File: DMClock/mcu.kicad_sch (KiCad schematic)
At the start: 23 parts, among them J7 Conn_01x01_Pin, J8 Conn_01x01_Pin, Q1 2SC1815, Q2 2SC1815, SW1 SW_Push, SW10 SW_Push, SW3 SW_SP3T (mode select), SW7 SW_Push, SW8 SW_Push, SW9 SW_Push, U1 PIC16F18346-P, U2 DS3231SN_

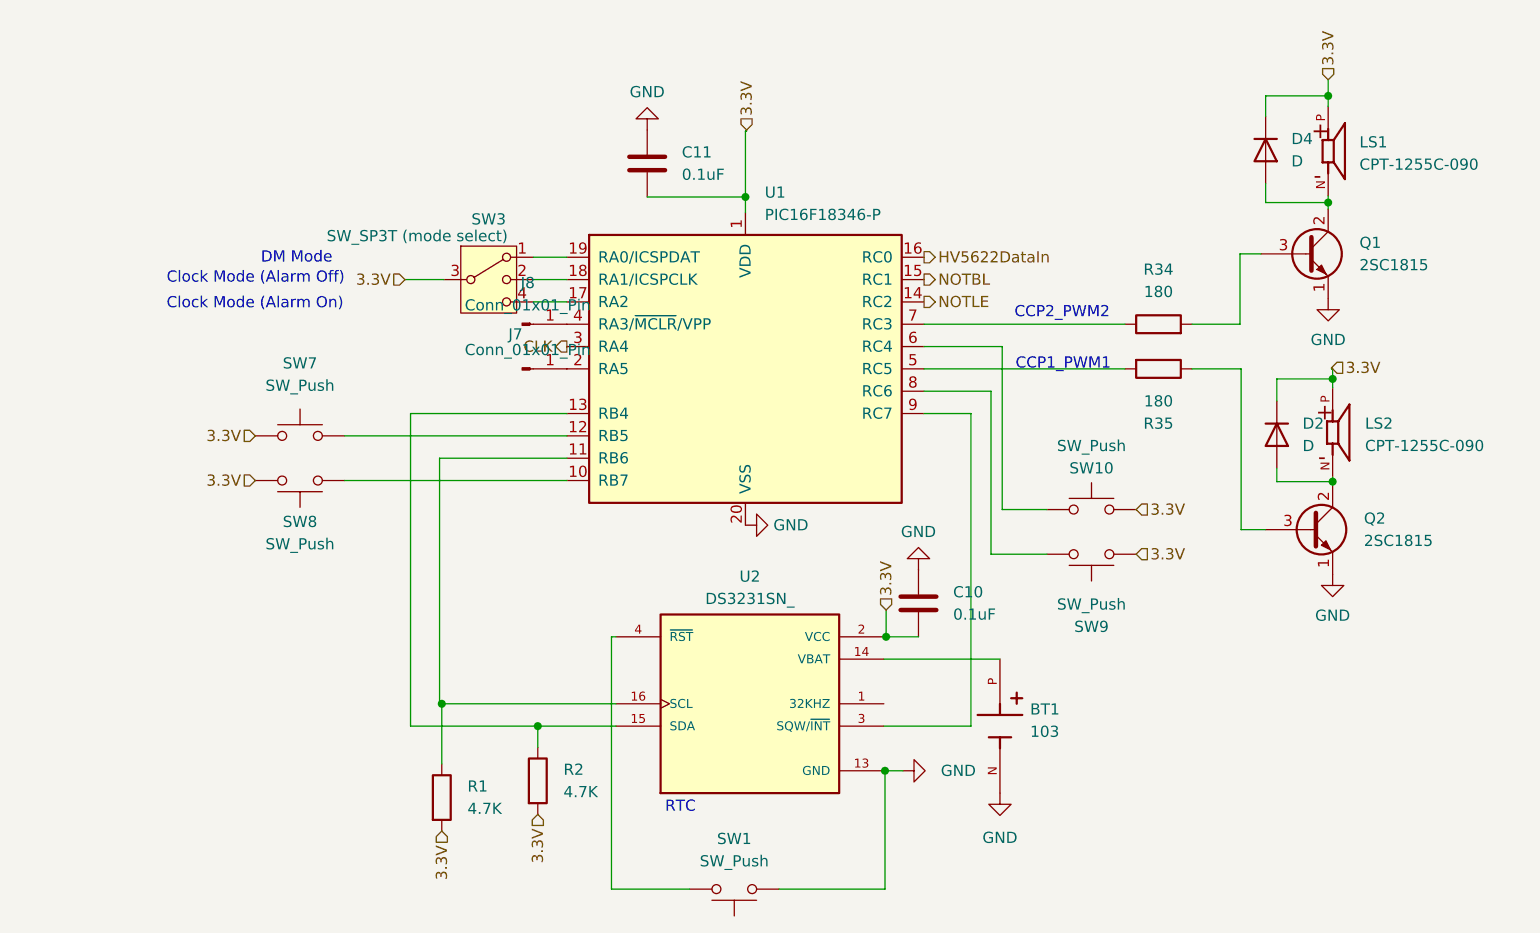
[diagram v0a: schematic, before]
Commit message: finished v.1
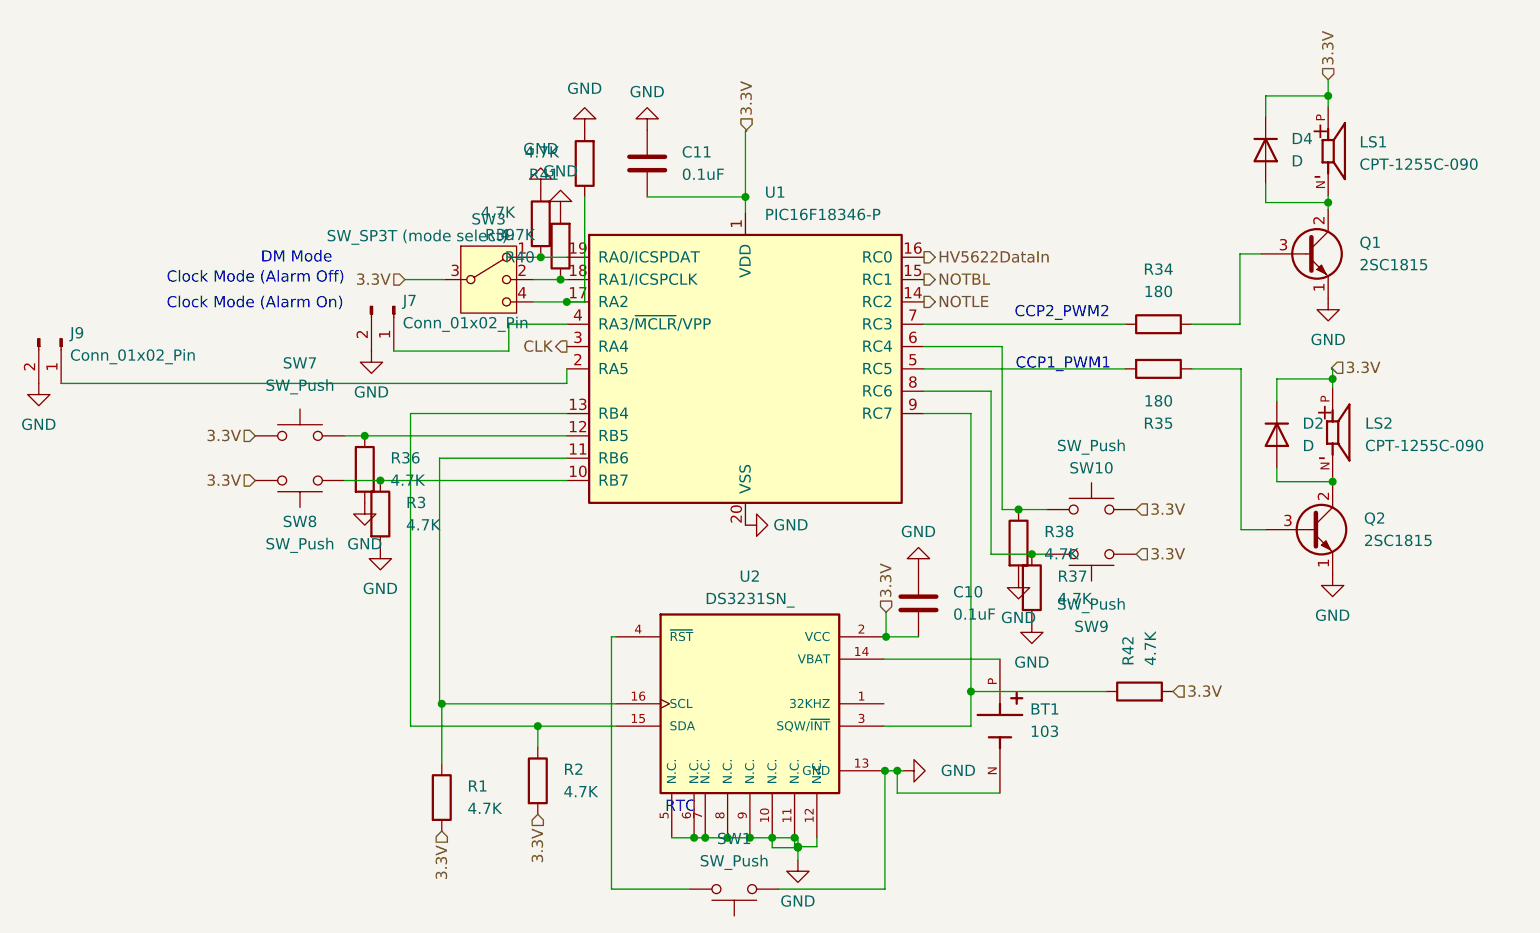
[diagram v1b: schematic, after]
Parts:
- removed J7, J8: Conn_01x01_Pin, Connector_PinSocket_2.54mm:PinSocket_1x01_P2.54mm_Vertical, symbol Connector:Conn_01x01_Pin
- added J7, J9: Conn_01x02_Pin, Connector_PinSocket_2.54mm:PinSocket_1x02_P2.54mm_Vertical, symbol Connector:Conn_01x02_Pin
- added R3, R36, R37, R38, R39, R40, R41, R42: 4.7K, Resistor_THT:R_Axial_DIN0204_L3.6mm_D1.6mm_P2.54mm_Vertical, symbol Device:R
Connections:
- net 3.3V: now also C10.1, U2.2 (VCC), R42.2
- net GND: now also U2.10 (N.C.), U2.11 (N.C.), U2.12 (N.C.), U2.5 (N.C.), U2.6 (N.C.), U2.7 (N.C.), U2.8 (N.C.), U2.9 (N.C.), J7.2 (Pin_2), J9.2 (Pin_2), R3.2, R36.2, R37.2, R38.2, R39.2, R40.2, R41.2
- net at SW10.1, U1.6 (RC4): now also R38.1
- net at U1.9 (RC7), U2.3 (SQW/~{INT}): now also R42.1
- net at SW8.1, U1.10 (RB7): now also R3.1
- net at U1.2 (RA5): now also J9.1 (Pin_1)
- net at U1.4 (RA3/~{MCLR}/VPP): now also J7.1 (Pin_1)
- net at SW9.2, U1.8 (RC6): now also R37.1
- net at SW7.2, U1.12 (RB5): now also R36.1
- net at SW3.4, U1.17 (RA2): now also R41.1
- net at SW3.2, U1.18 (RA1/ICSPCLK): now also R40.1
- net at SW3.1, U1.19 (RA0/ICSPDAT): now also R39.1

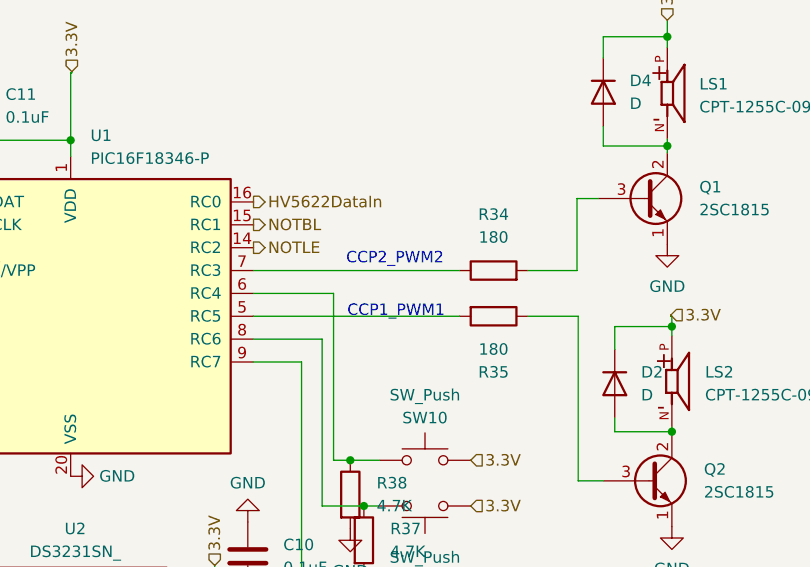
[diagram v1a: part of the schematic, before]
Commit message: initial mpe files
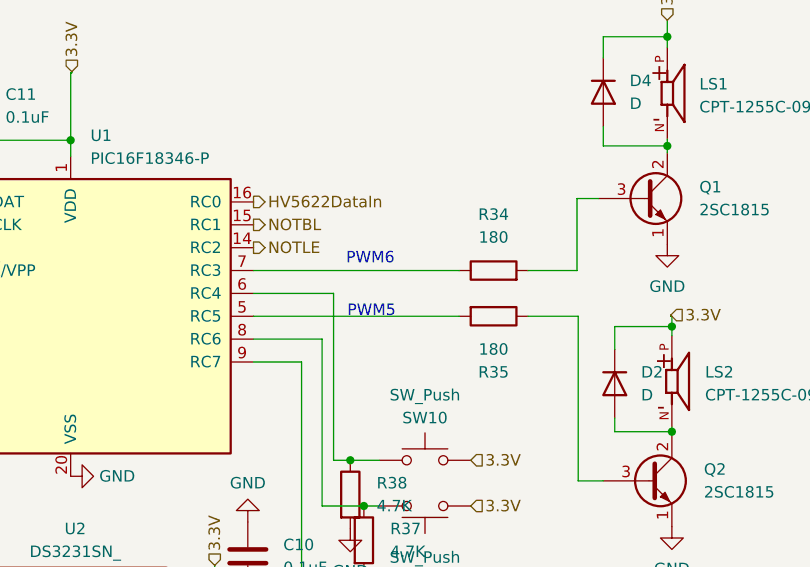
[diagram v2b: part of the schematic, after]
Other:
- note added: "PWM5"
- note added: "PWM6"
- note removed: "CCP1_PWM1"
- note removed: "CCP2_PWM2"
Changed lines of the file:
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@@
     (effects (font (size 1.27 1.27)) (justify right bottom))
   )
-  (text "CCP2_PWM2" (at 155.702 64.135 0)
+  (text "PWM6" (at 155.702 64.135 0)
     (effects (font (size 1.27 1.27)) (justify left bottom))
   )
-  (text "CCP1_PWM1" (at 155.829 69.977 0)
+  (text "PWM5" (at 155.829 69.977 0)
     (effects (font (size 1.27 1.27)) (justify left bottom))
   )
